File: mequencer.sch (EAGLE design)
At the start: 75 parts, among them IC1 NE555D, IC10 LF353D, IC11 NE555D, IC12 NE555D, IC2 4163D, IC3 74HC85D, IC4 4051D, IC5 4051D, IC6 74HCT04D, IC7 4051D, IC8 4051D, IC9 LF353D, U1 74LVC1G08SE-7

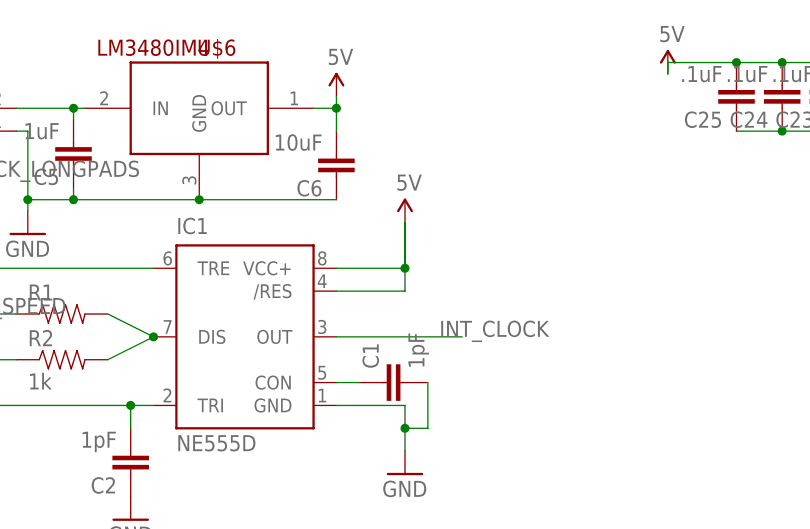
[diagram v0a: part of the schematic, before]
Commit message: Moving shit around
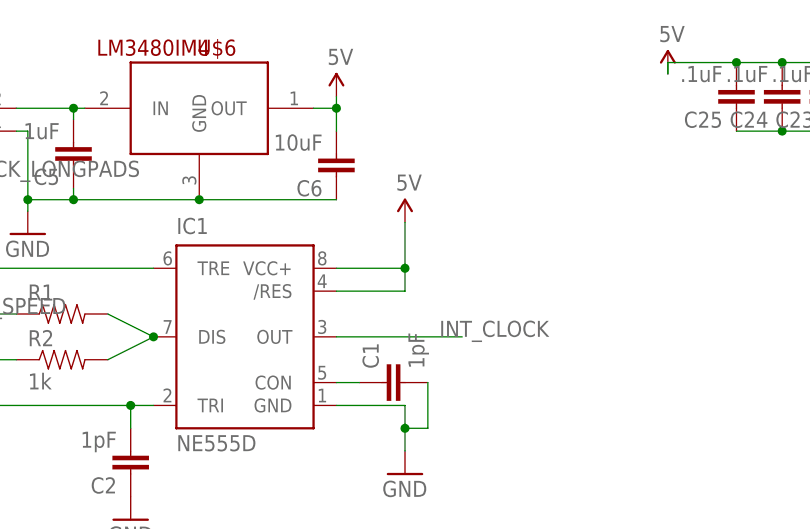
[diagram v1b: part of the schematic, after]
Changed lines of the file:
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@@
 <segment>
 <pinref part="SUPPLY2" gate="G$1" pin="5V"/>
-<wire x1="63.5" y1="165.1" x2="63.5" y2="160.02" width="0.1524" layer="91"/>
 <pinref part="IC1" gate="G$1" pin="VCC+"/>
 <wire x1="63.5" y1="160.02" x2="55.88" y2="160.02" width="0.1524" layer="91"/>
